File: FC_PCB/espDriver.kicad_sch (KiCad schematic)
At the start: 7 parts, among them J1 PWM1, J4 PWM2, J5 PWM3, J6 PWM4, J7 I2C, J8 UART, J9 SPI

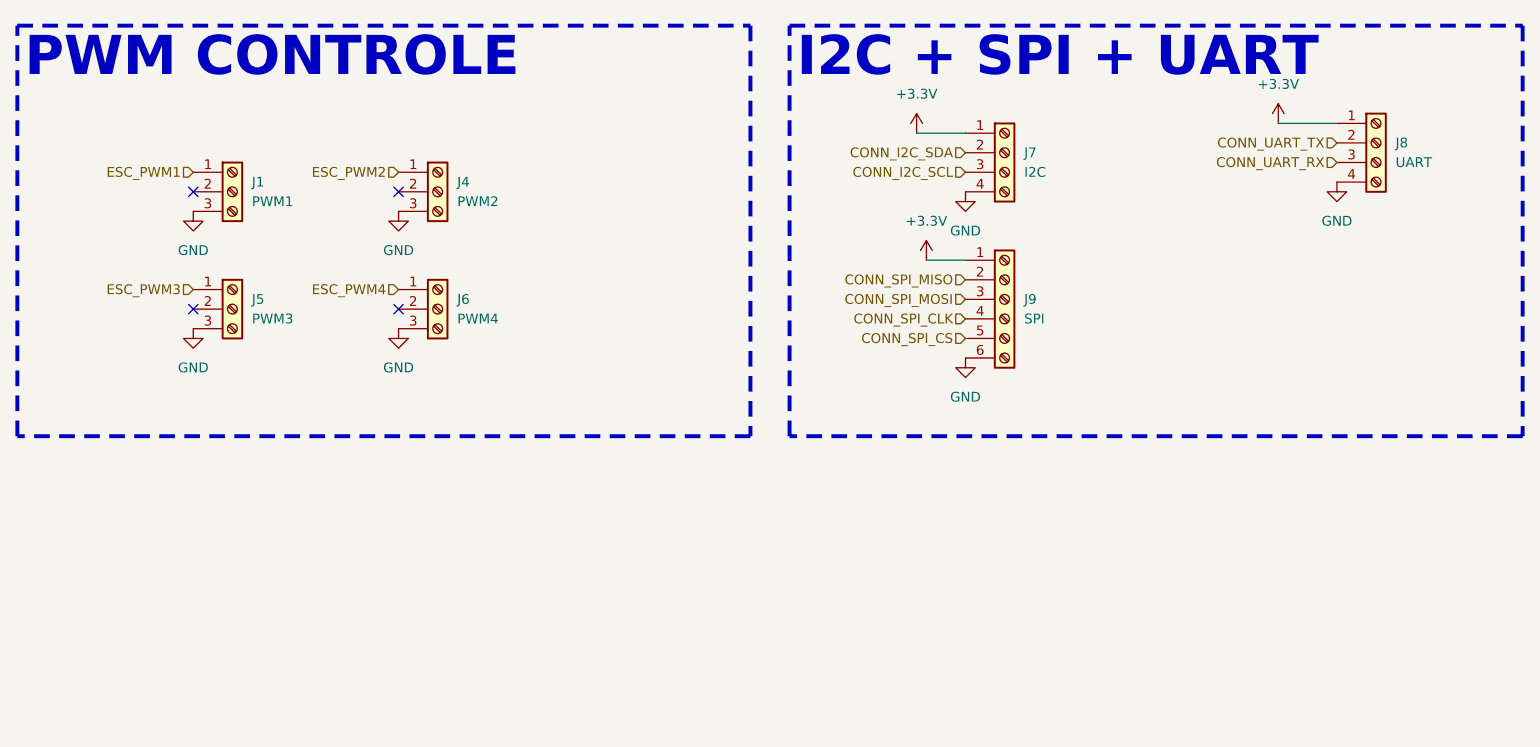
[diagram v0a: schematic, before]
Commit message: Commit final hard
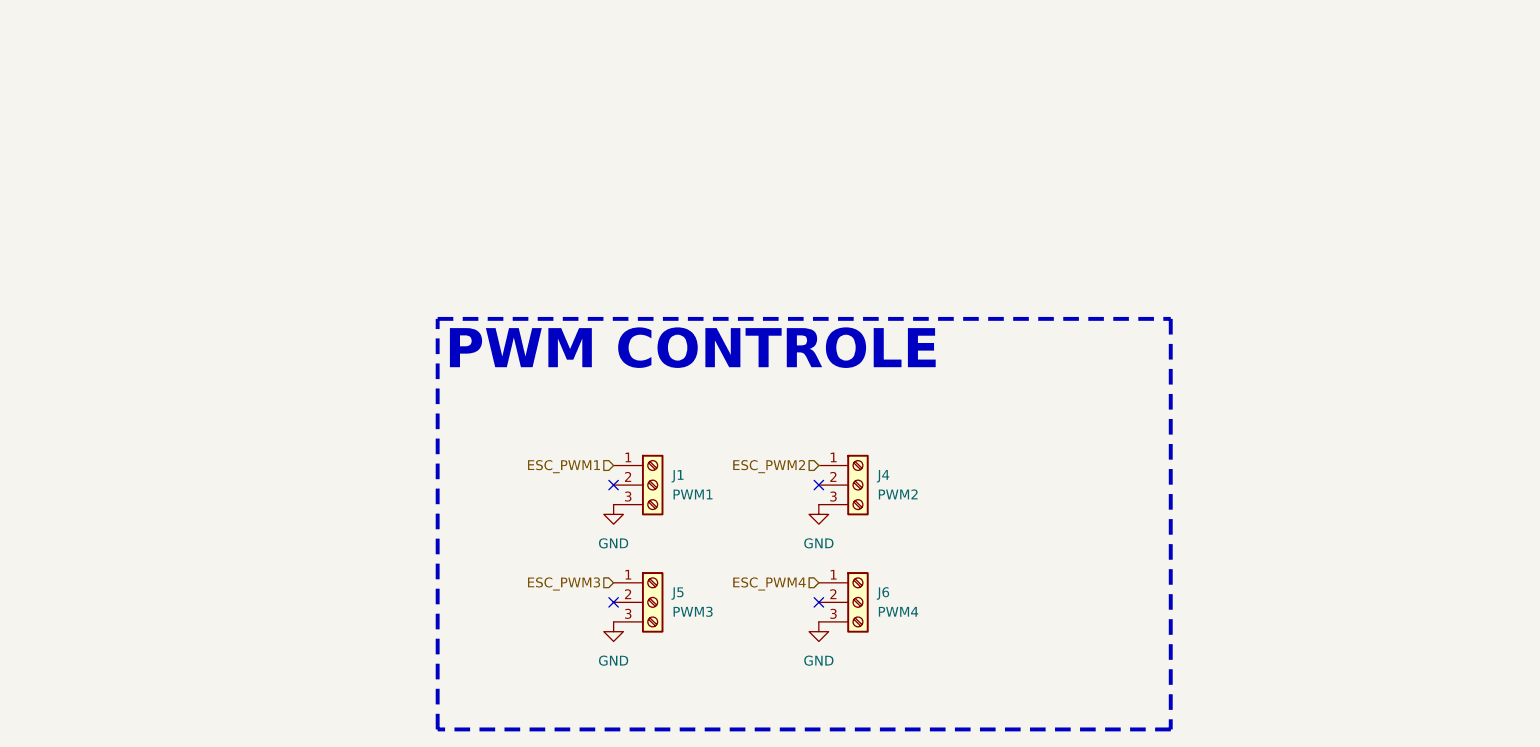
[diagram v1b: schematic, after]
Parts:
- removed J7: I2C, Connector_JST:JST_EH_B4B-EH-A_1x04_P2.50mm_Vertical, symbol Connector:Screw_Terminal_01x04
- removed J8: UART, Connector_JST:JST_EH_B4B-EH-A_1x04_P2.50mm_Vertical, symbol Connector:Screw_Terminal_01x04
- removed J9: SPI, Connector_JST:JST_EH_B6B-EH-A_1x06_P2.50mm_Vertical, symbol Connector:Screw_Terminal_01x06
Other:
- moved on the sheet: J1, J4, J5, J6
